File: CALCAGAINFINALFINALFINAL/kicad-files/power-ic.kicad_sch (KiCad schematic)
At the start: 15 parts, among them J2 USB_C_Receptacle_USB2.0_16P, J4 Conn_01x02, U2 TPS73733DCQR, U5 TP4056-42-ESOP8

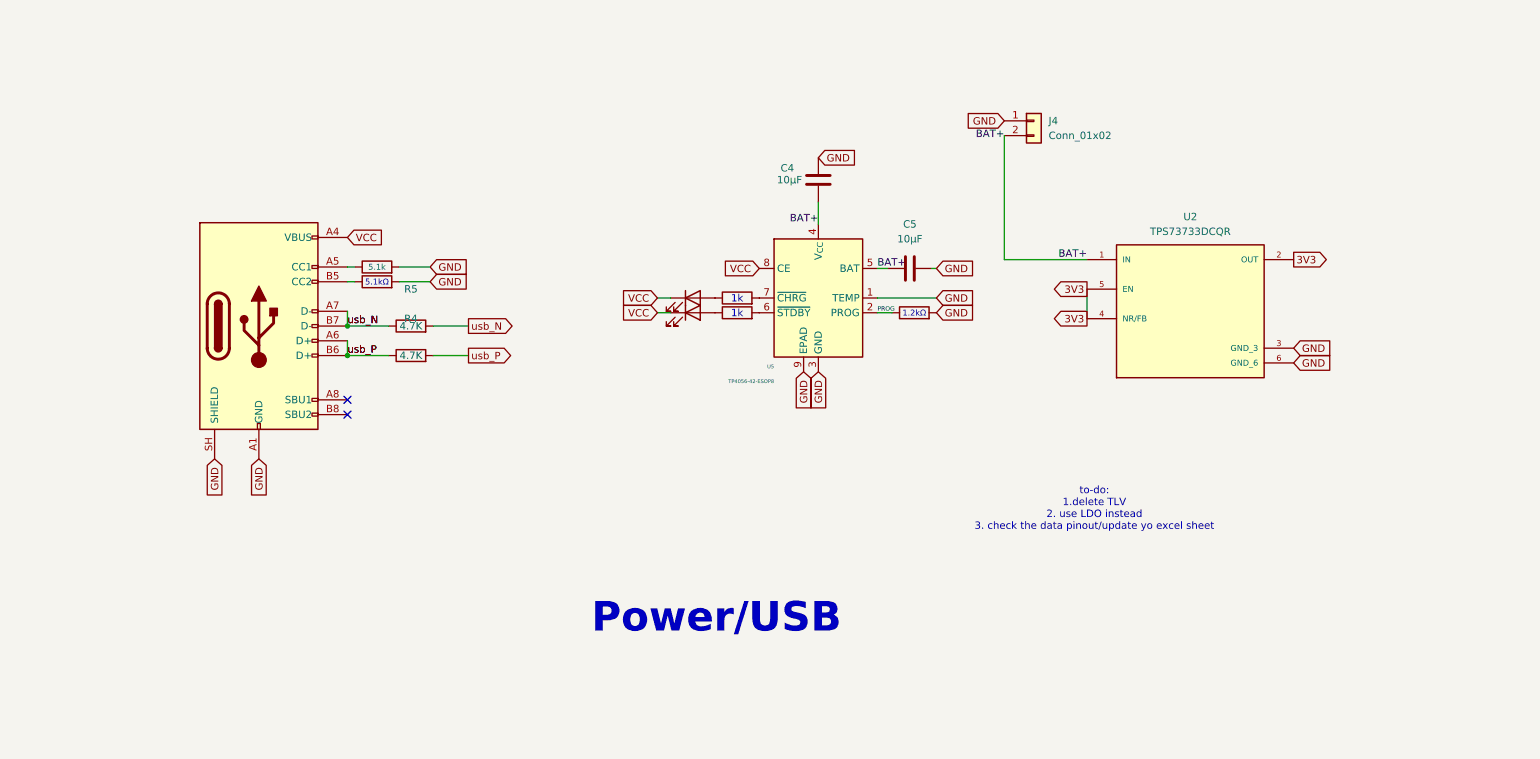
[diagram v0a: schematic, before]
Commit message: yo chat this actually for reals the order now im ordering it and neva openin kicad again ong
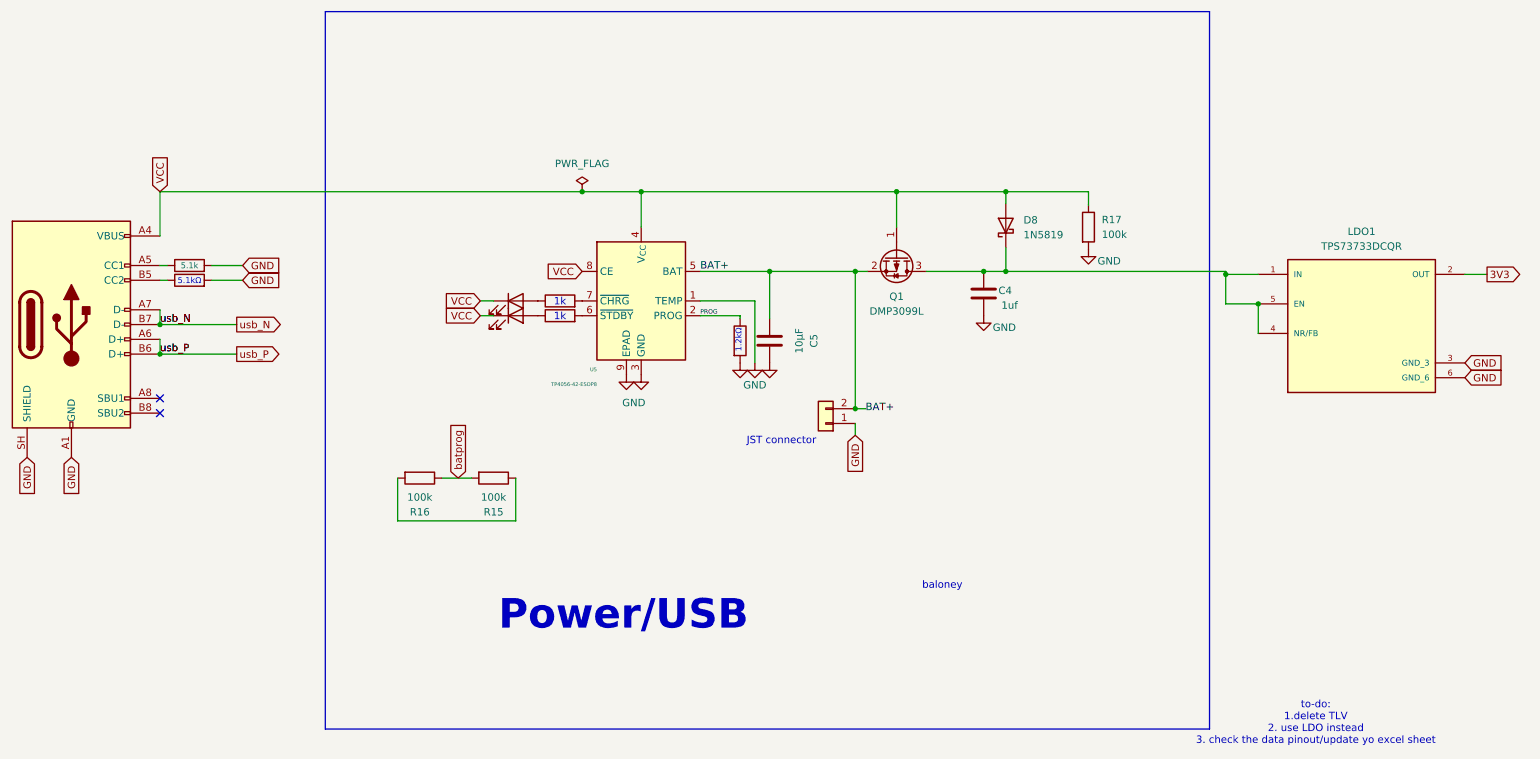
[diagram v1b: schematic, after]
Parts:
- removed R4, R5: 4.7K, symbol Device:R
- added D8: 1N5819, Diode_THT:D_DO-41_SOD81_P10.16mm_Horizontal, symbol Diode:1N5819
- added Q1: DMP3099L, Package_TO_SOT_SMD:SOT-23, symbol Transistor_FET:DMP3099L
- added R15, R16, R17: 100k, symbol Device:R
- C4: value 10µF -> 1uf; footprint Capacitor_SMD:C_0603_1608Metric -> (none); KiLib_Generator SMD_2terminal_chip_molded -> (none); LCSC C7171 -> (none)
- renumbered U2 to LDO1
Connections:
- net 3V3: no longer LDO1.4 (NR/FB), LDO1.5 (EN)
- net BAT+: now also Q1.2 (S); no longer C4.2, LDO1.1 (IN), U5.4 (V_{CC})
- net GND: now also C4.2, R17.2; no longer C4.1
- net VCC: now also U5.4 (V_{CC}), D8.2 (A), Q1.1 (G), R17.1
- new net: R15.1, R16.2
- new net: C4.1, D8.1 (K), LDO1.1 (IN), LDO1.4 (NR/FB), LDO1.5 (EN), Q1.3 (D)
- new net batprog: R15.2, R16.1
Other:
- note added: "JST connector"
- note added: "baloney"
- moved on the sheet: C5, LDO1, U5
